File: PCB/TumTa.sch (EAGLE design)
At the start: 20 parts

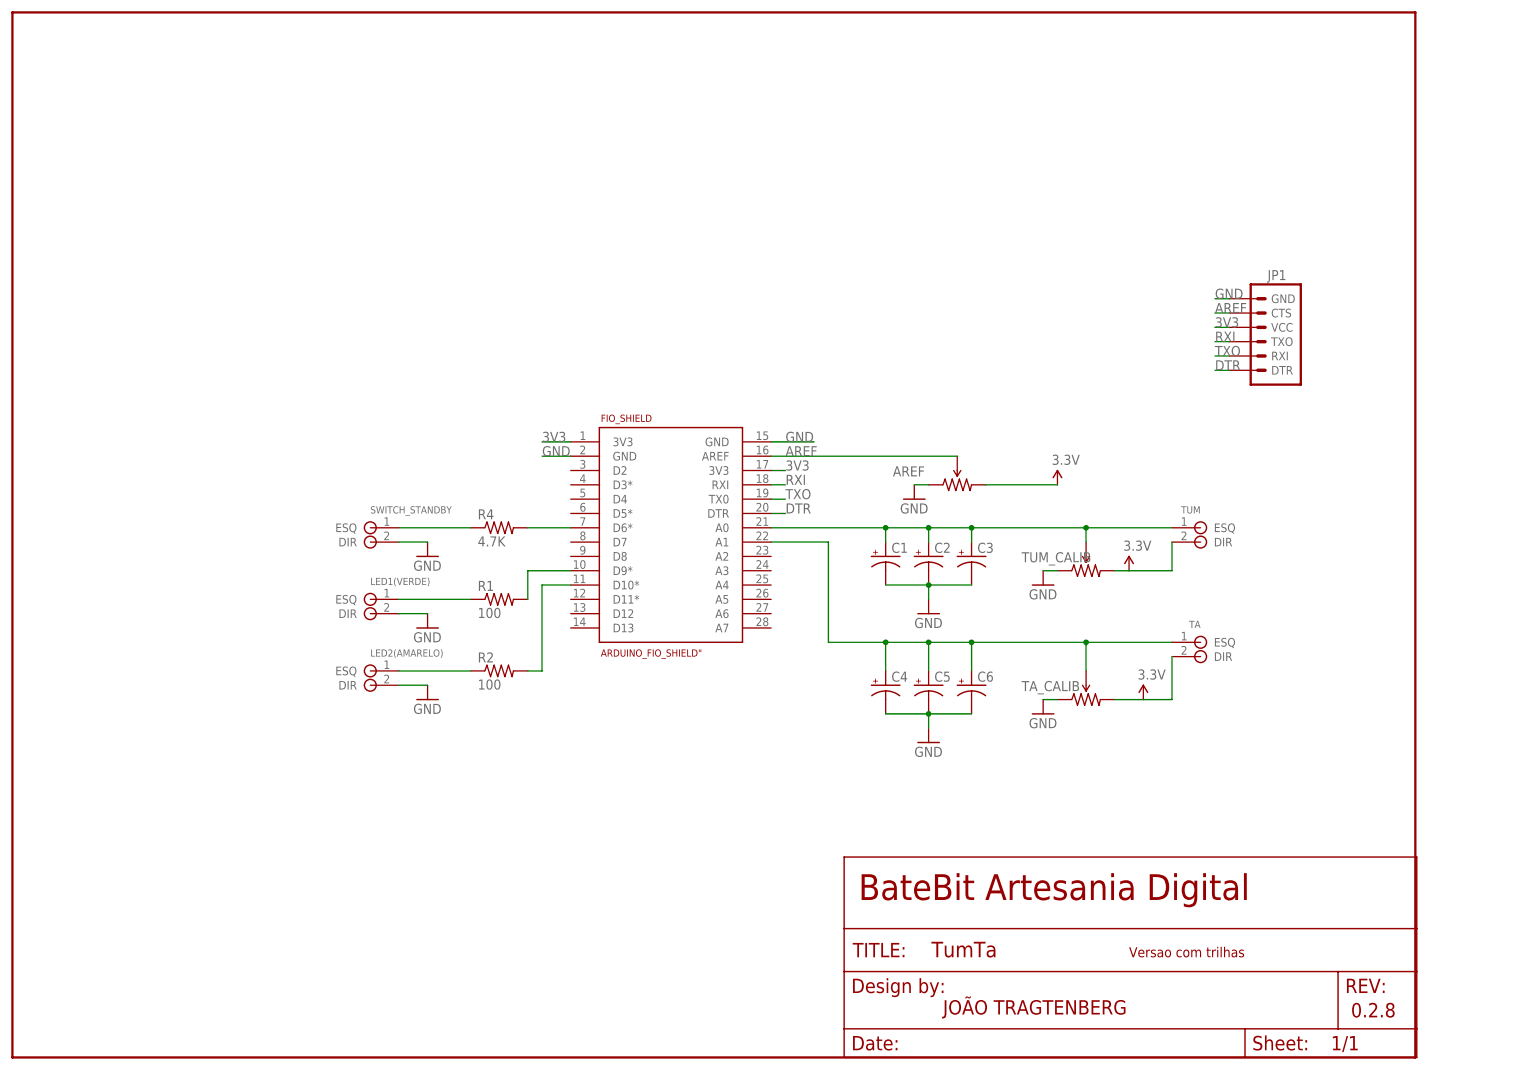
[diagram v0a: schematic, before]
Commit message: v0_2_9
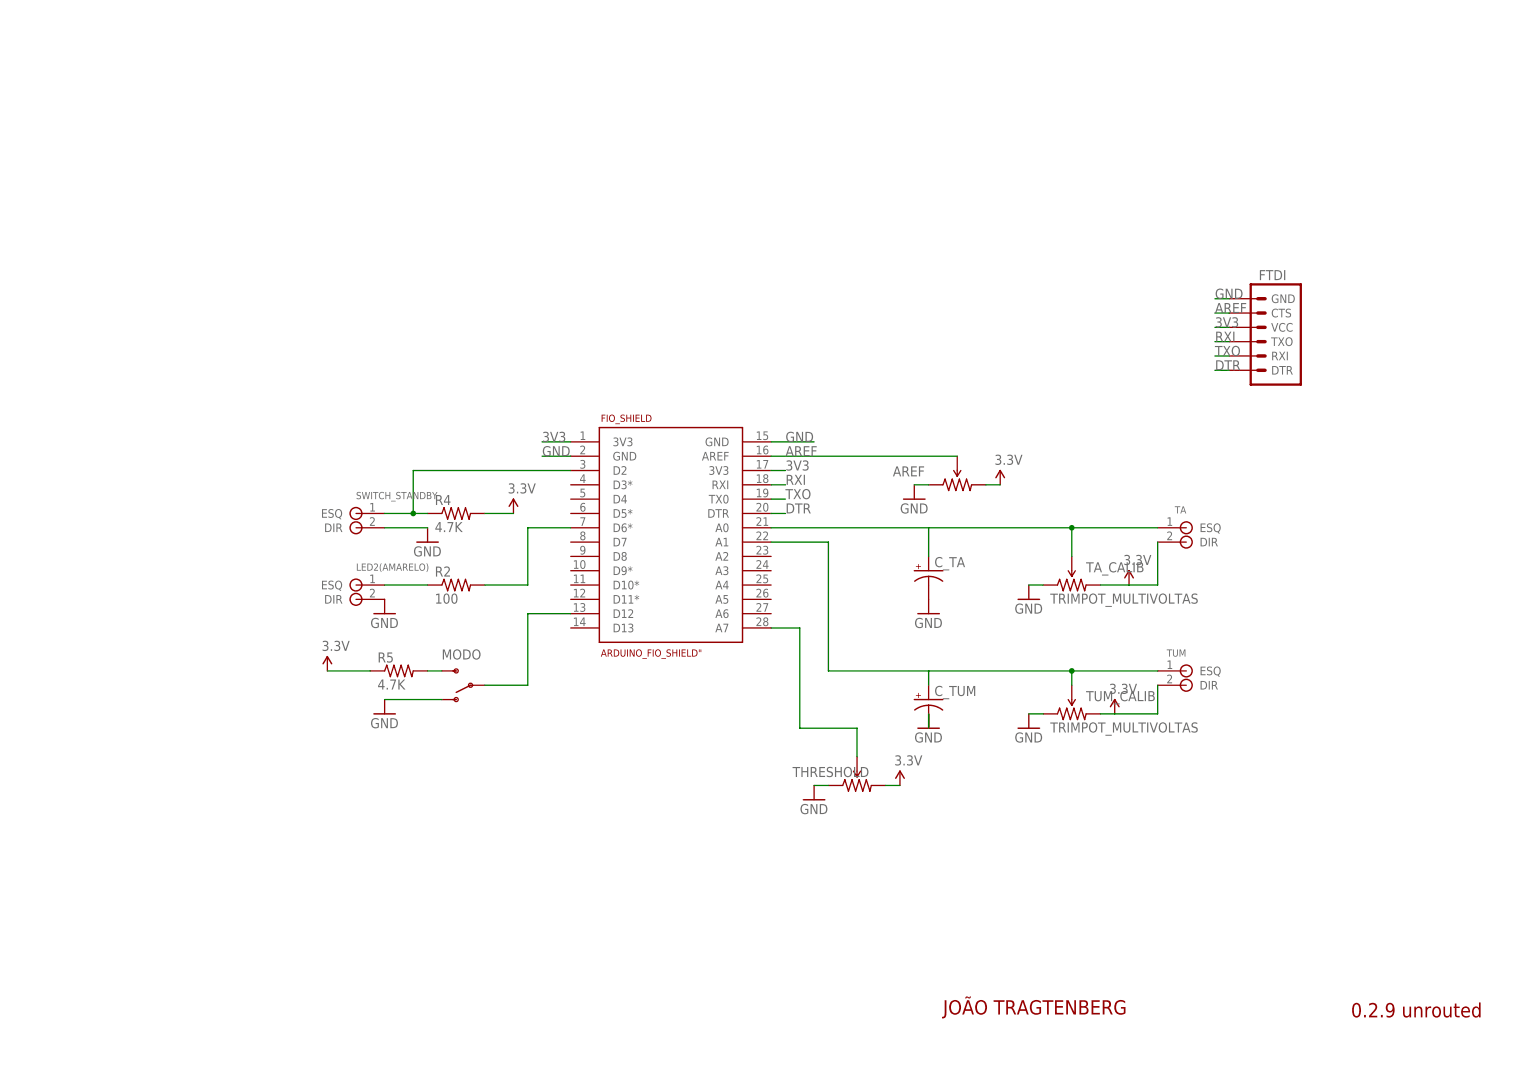
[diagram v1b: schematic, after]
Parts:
- removed C1, C2, C3, C4, C5, C6: (no value), SparkFun-Passives:CAP_POLPTH2
- removed FL1: FRAME-LETTER_BATEBIT, SparkFun-Retired:FRAME-LETTER_BATEBIT
- removed LED1(VERDE): SCREWTERMINAL-25MM, SparkFun-Connectors:SCREWTERMINAL-25MM
- removed R1: 100, SparkFun-Resistors:10OHM-1/10W-1%(0603)SMD
- added C_TA, C_TUM: (no value), SparkFun-Passives:CAP_POLPTH2
- added MODO: (no value), SparkFun-Electromechanical:SWITCH-SPDTPTH
- added R5: 4.7K, SparkFun-Resistors:4.7KOHM-1/10W-1%(0603)
- added THRESHOLD: (no value), SparkFun-Electromechanical:TRIMPOTBR
- TA_CALIB, TUM_CALIB: value (none) -> TRIMPOT_MULTIVOLTAS; device SparkFun-Electromechanical:TRIMPOTBR -> SparkFun-Electromechanical:TRIMPOT_MULTIVOLTAS
- renumbered JP1 to FTDI
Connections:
- removed net 3.3V: TA.DIR, TA_CALIB.CW, TUM.DIR, TUM_CALIB.CW
- removed net D6: FIO_SHIELD.D6*, R4.2
- removed net D9: FIO_SHIELD.D9*, R1.2
- new net N$1: FIO_SHIELD.A7, THRESHOLD.WIPER
- new net N$4: MODO.S, R5.2
- net 3V3: now also R4.2, R5.1, TA.DIR, TA_CALIB.CW, THRESHOLD.CW, TUM.DIR, TUM_CALIB.CW
- net A0: now also C_TUM.+, FIO_SHIELD.A1; no longer C1.+, C2.+, C3.+, FIO_SHIELD.A0
- net A1: now also C_TA.+, FIO_SHIELD.A0; no longer C4.+, C5.+, C6.+, FIO_SHIELD.A1
- net D10: now also FIO_SHIELD.D6*; no longer FIO_SHIELD.D10*
- net GND: now also C_TA.-, C_TUM.-, MODO.O, THRESHOLD.CCW; no longer C1.-, C2.-, C3.-, C4.-, C5.-, C6.-, LED1(VERDE).DIR
- net N$2: now also FIO_SHIELD.D2
- net N$3: now also FIO_SHIELD.D12, MODO.P; no longer LED1(VERDE).ESQ, R1.1
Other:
- note added: "0.2.9 unrouted"
- note removed: "0.2.8"
- note removed: "Versao com trilhas"
- moved on the sheet: LED2(AMARELO), R2, R4, SWITCH_STANDBY, TA, TUM

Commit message: v1_0_0
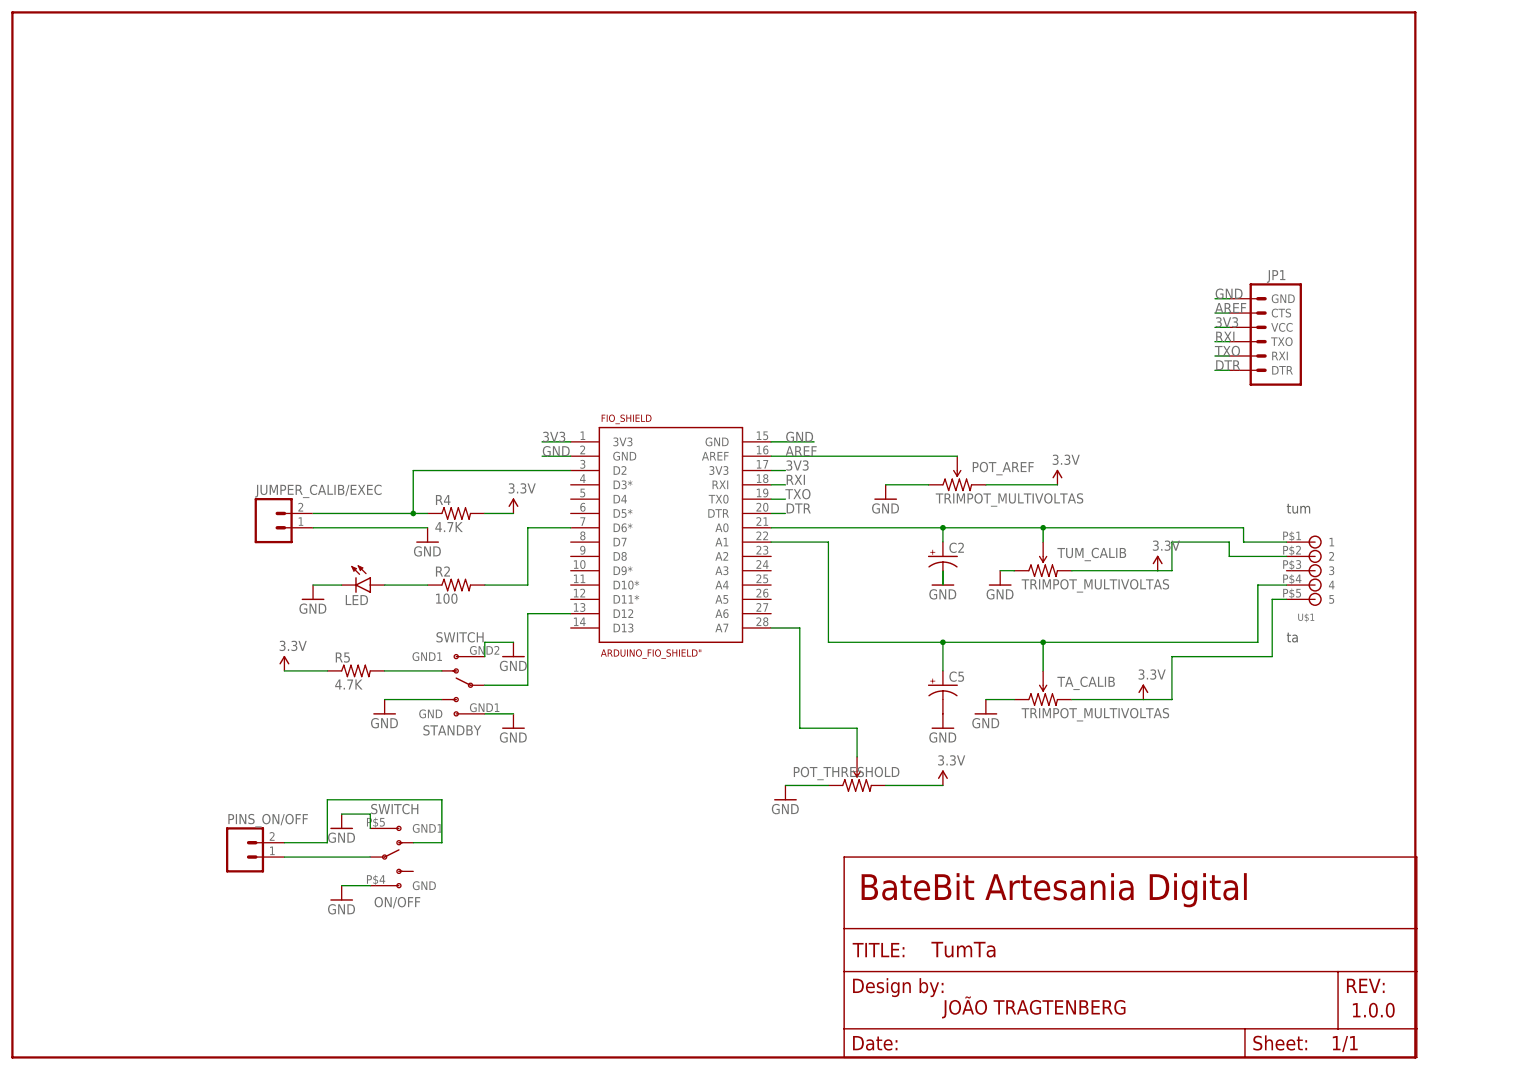
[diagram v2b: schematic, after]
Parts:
- removed AREF: (no value), SparkFun-Electromechanical:TRIMPOTBR
- removed C_TA, C_TUM: (no value), SparkFun-Passives:CAP_POLPTH2
- removed LED2(AMARELO), SWITCH_STANDBY, TA, TUM: SCREWTERMINAL-25MM, SparkFun-Connectors:SCREWTERMINAL-25MM
- removed MODO: (no value), SparkFun-Electromechanical:SWITCH-SPDTPTH
- added C2, C5: (no value), SparkFun-Passives:CAP_POLPTH2
- added FL1: FRAME-LETTER_BATEBIT, SparkFun-Retired:FRAME-LETTER_BATEBIT
- added JUMPER_CALIB/EXEC, PINS_ON/OFF: (no value), SparkFun-Connectors:M02PTH
- added LED: (no value), SparkFun-LED:LED-GREEN5MM_THRU
- added ON/OFF: SWITCH, SparkFun-Electromechanical:SWITCH-SPDT-COM-GND3PIN
- added POT_AREF: TRIMPOT_MULTIVOLTAS, SparkFun-Electromechanical:TRIMPOT_MULTIVOLTAS
- added STANDBY: SWITCH, SparkFun-Electromechanical:SWITCH-SPDT-COM-GND6PIN
- added U$1: SCREWTERMINAL-5, SparkFun-Connectors:SCREWTERMINAL-5
- renumbered FTDI to JP1, THRESHOLD to POT_THRESHOLD
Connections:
- new net 3.3V: POT_THRESHOLD.CW
- new net N$6: ON/OFF.O, PINS_ON/OFF.2
- new net N$8: ON/OFF.P, PINS_ON/OFF.1
- net 3V3: now also POT_AREF.CW, U$1.2, U$1.5; no longer AREF.CW, POT_THRESHOLD.CW, TA.DIR, TUM.DIR
- net A0: now also C2.+, FIO_SHIELD.A0, U$1.1; no longer C_TUM.+, FIO_SHIELD.A1, TUM.ESQ
- net A1: now also C5.+, FIO_SHIELD.A1, U$1.4; no longer C_TA.+, FIO_SHIELD.A0, TA.ESQ
- net AREF: now also POT_AREF.WIPER; no longer AREF.WIPER
- net GND: now also C2.-, C5.-, JUMPER_CALIB/EXEC.1, LED.C, ON/OFF.GND, ON/OFF.GND1, POT_AREF.CCW, STANDBY.GND, STANDBY.GND1, STANDBY.S; no longer AREF.CCW, C_TA.-, C_TUM.-, LED2(AMARELO).DIR, MODO.O, SWITCH_STANDBY.DIR
- net N$2: now also JUMPER_CALIB/EXEC.2; no longer SWITCH_STANDBY.ESQ
- net N$3: now also STANDBY.P; no longer MODO.P
- net N$4: now also STANDBY.O; no longer MODO.S
- net N$7: now also LED.A; no longer LED2(AMARELO).ESQ
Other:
- note added: "1.0.0"
- note added: "ta"
- note added: "tum"
- note removed: "0.2.9 unrouted"
- moved on the sheet: R5, TA_CALIB, TUM_CALIB
